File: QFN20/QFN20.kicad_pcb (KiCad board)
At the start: 2 copper layers, 25.7 x 13 mm, 9 parts, among them J1 Conn_01x10, J2 Conn_02x10_Counter_Clockwise, J3 Conn_01x10, J4 Conn_02x10_Counter_Clockwise, J5 Conn_01x03

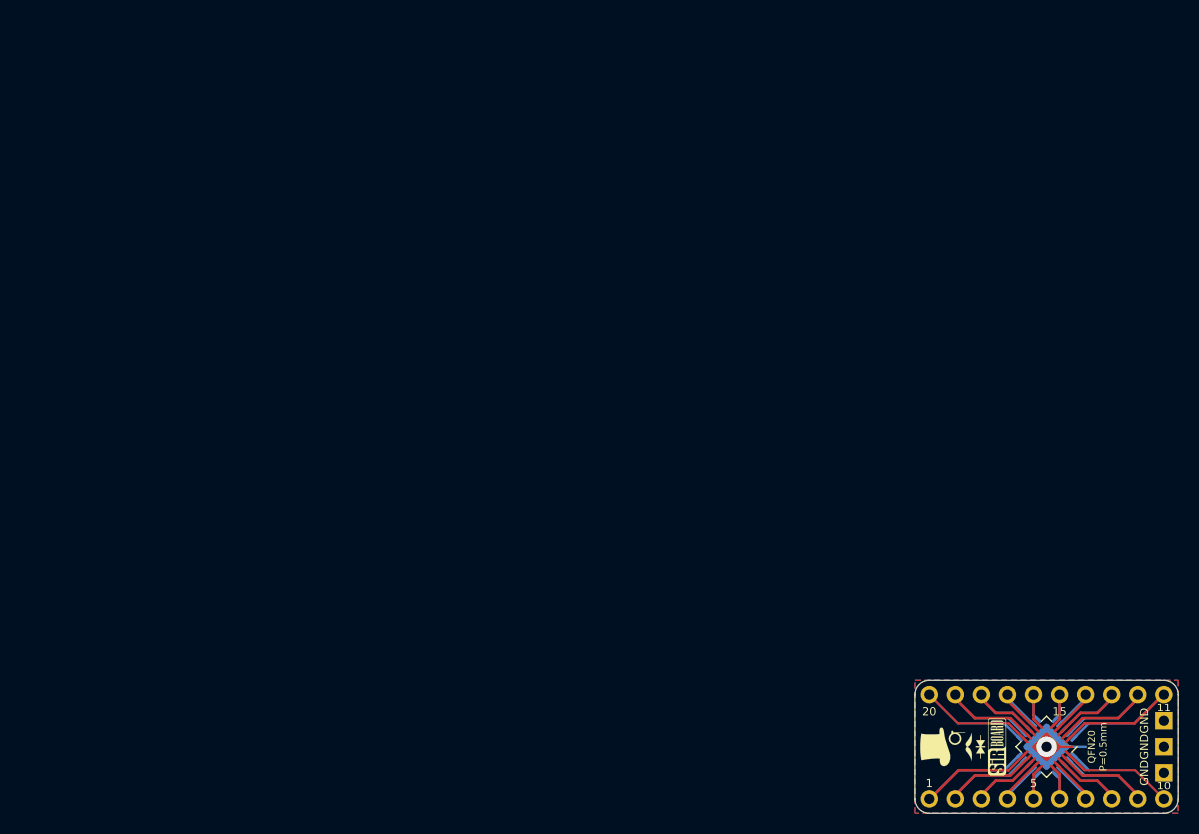
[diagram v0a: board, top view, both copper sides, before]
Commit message: Page Settings Updated
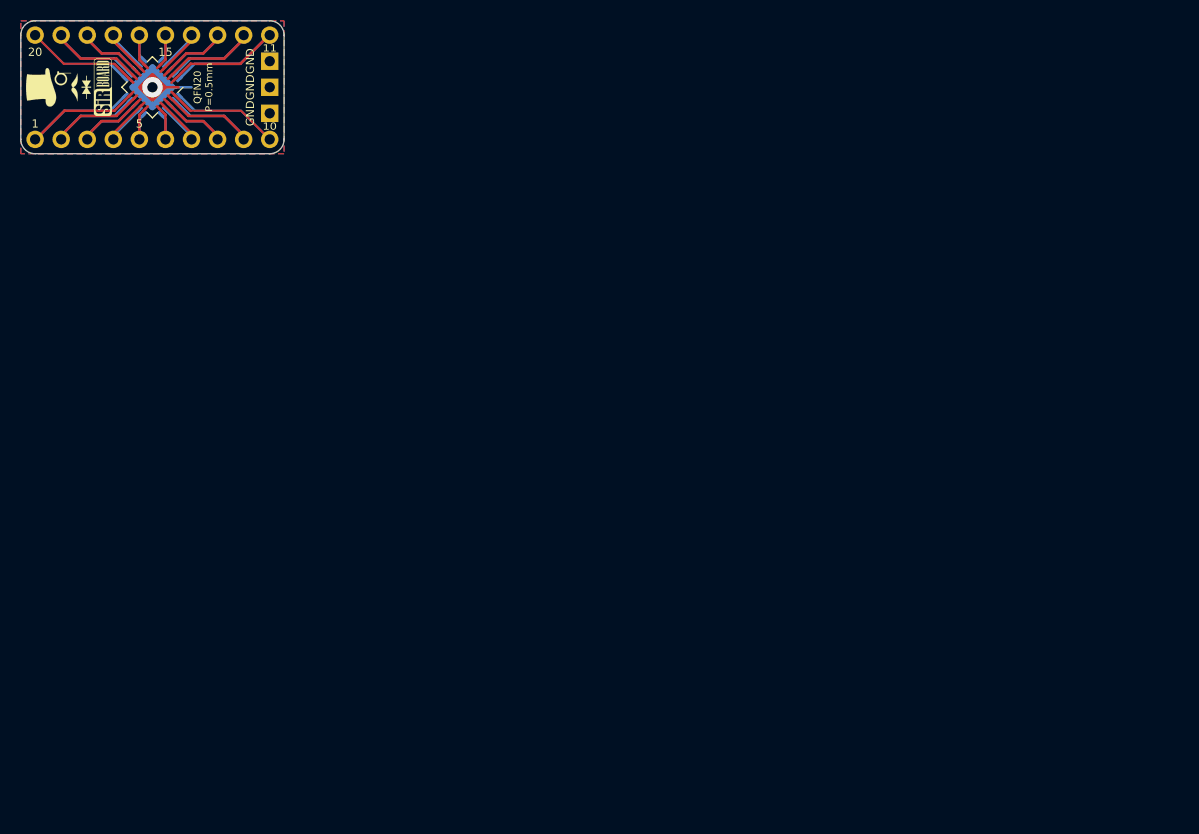
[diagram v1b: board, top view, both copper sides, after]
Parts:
- moved G*** 108.3 mm to (61.2, 42.2)
- moved G*** 108.3 mm to (61.1, 42.0)
- moved G*** 108.3 mm to (65.5, 42.2) (x2)
- moved J1 108.3 mm to (81.8, 37.1)
- moved J3 108.3 mm to (81.8, 47.2)
- moved J5 108.3 mm to (81.8, 39.6)
- moved J2 108.3 mm to (70.4, 42.2)
- moved J4 108.3 mm to (70.4, 42.2)

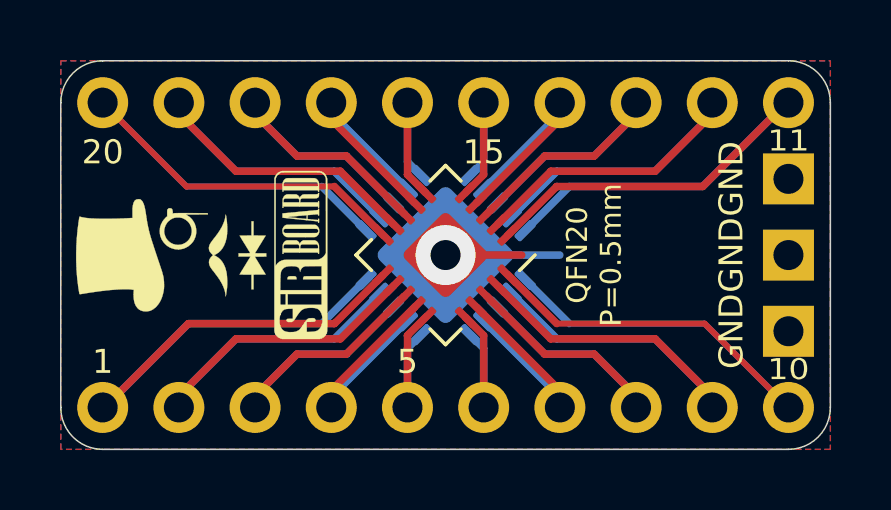
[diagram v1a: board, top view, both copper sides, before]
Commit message: Board Updates
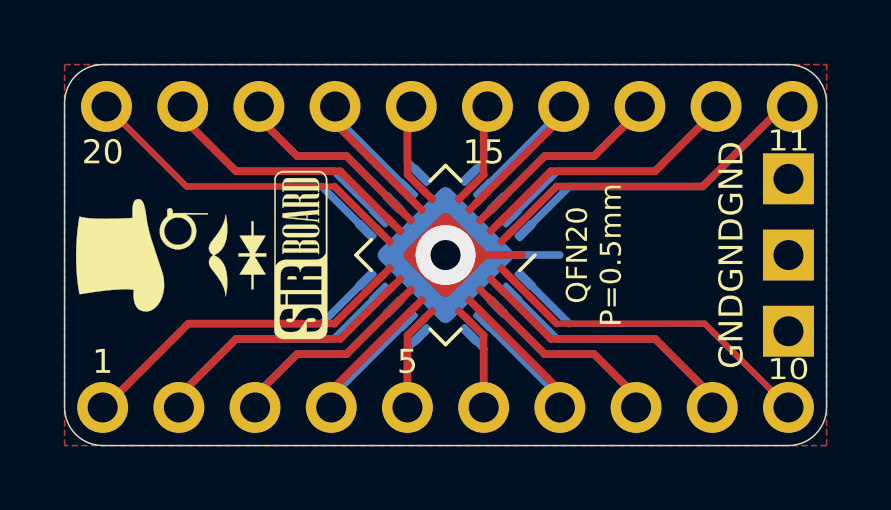
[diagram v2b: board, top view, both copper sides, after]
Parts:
- moved J1 0.18 mm to (81.9, 37.2)
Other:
- board size 25.7 x 13 mm -> 25.4 x 12.7 mm
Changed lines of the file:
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@@
   )
   (module Connector_PinHeader_2.54mm:PinHeader_1x10_P2.54mm_Vertical (layer F.Cu)
-    (at 81.788 37.084 270)
+    (at 81.915 37.211 270)
     (descr "Through hole straight pin header, 1x10, 2.54mm pitch, single row")
     (tags "Through hole pin header THT 1x10 2.54mm single row")
@@
     )
   )
+  (gr_arc (start 81.788 37.084) (end 83.058 37.084) (angle -90) (layer Edge.Cuts) (width 0.05))
+  (gr_arc (start 81.788 47.244) (end 81.788 48.514) (angle -90) (layer Edge.Cuts) (width 0.05))
+  (gr_arc (start 58.928 47.244) (end 57.658 47.244) (angle -90) (layer Edge.Cuts) (width 0.05))
+  (gr_arc (start 58.928 37.084) (end 58.928 35.814) (angle -90) (layer Edge.Cuts) (width 0.05))
   (dimension 22.86 (width 0.15) (layer Dwgs.User)
     (gr_text "22.860 mm" (at 70.358 32.609) (layer Dwgs.User)
@@
     (arrow2b (pts (xy 58.928 33.909) (xy 60.054504 33.322579)))
   )
-  (dimension 25.654 (width 0.15) (layer Dwgs.User)
-    (gr_text "25.654 mm" (at 70.358 29.942) (layer Dwgs.User)
+  (dimension 25.4 (width 0.15) (layer Dwgs.User)
+    (gr_text "25.400 mm" (at 70.358 30.069) (layer Dwgs.User)
       (effects (font (size 1 1) (thickness 0.15)) hide)
     )
-    (feature1 (pts (xy 83.185 35.687) (xy 83.185 30.655579)))
-    (feature2 (pts (xy 57.531 35.687) (xy 57.531 30.655579)))
-    (crossbar (pts (xy 57.531 31.242) (xy 83.185 31.242)))
-    (arrow1a (pts (xy 83.185 31.242) (xy 82.058496 31.828421)))
-    (arrow1b (pts (xy 83.185 31.242) (xy 82.058496 30.655579)))
-    (arrow2a (pts (xy 57.531 31.242) (xy 58.657504 31.828421)))
-    (arrow2b (pts (xy 57.531 31.242) (xy 58.657504 30.655579)))
+    (feature1 (pts (xy 83.058 37.084) (xy 83.058 30.782579)))
+    (feature2 (pts (xy 57.658 37.084) (xy 57.658 30.782579)))
+    (crossbar (pts (xy 57.658 31.369) (xy 83.058 31.369)))
+    (arrow1a (pts (xy 83.058 31.369) (xy 81.931496 31.955421)))
+    (arrow1b (pts (xy 83.058 31.369) (xy 81.931496 30.782579)))
+    (arrow2a (pts (xy 57.658 31.369) (xy 58.784504 31.955421)))
+    (arrow2b (pts (xy 57.658 31.369) (xy 58.784504 30.782579)))
   )
   (gr_text 11 (at 81.788 45.974 180) (layer B.SilkS)
@@
     (arrow2b (pts (xy 55.372 47.244) (xy 54.785579 46.117496)))
   )
-  (dimension 12.954 (width 0.15) (layer Dwgs.User)
-    (gr_text "12.954 mm" (at 50.77 42.164 90) (layer Dwgs.User)
+  (dimension 12.7 (width 0.15) (layer Dwgs.User)
+    (gr_text "12.700 mm" (at 51.278 42.164 90) (layer Dwgs.User)
       (effects (font (size 1 1) (thickness 0.15)) hide)
     )
-    (feature1 (pts (xy 57.531 35.687) (xy 51.483579 35.687)))
-    (feature2 (pts (xy 57.531 48.641) (xy 51.483579 48.641)))
-    (crossbar (pts (xy 52.07 48.641) (xy 52.07 35.687)))
-    (arrow1a (pts (xy 52.07 35.687) (xy 52.656421 36.813504)))
-    (arrow1b (pts (xy 52.07 35.687) (xy 51.483579 36.813504)))
-    (arrow2a (pts (xy 52.07 48.641) (xy 52.656421 47.514496)))
-    (arrow2b (pts (xy 52.07 48.641) (xy 51.483579 47.514496)))
+    (feature1 (pts (xy 58.928 35.814) (xy 51.991579 35.814)))
+    (feature2 (pts (xy 58.928 48.514) (xy 51.991579 48.514)))
+    (crossbar (pts (xy 52.578 48.514) (xy 52.578 35.814)))
+    (arrow1a (pts (xy 52.578 35.814) (xy 53.164421 36.940504)))
+    (arrow1b (pts (xy 52.578 35.814) (xy 51.991579 36.940504)))
+    (arrow2a (pts (xy 52.578 48.514) (xy 53.164421 47.387496)))
+    (arrow2b (pts (xy 52.578 48.514) (xy 51.991579 47.387496)))
   )
   (gr_text GND (at 79.883 44.704 90) (layer B.SilkS)
@@
     (effects (font (size 0.7 0.7) (thickness 0.15)))
   )
-  (gr_line (start 57.531 37.084) (end 57.531 47.244) (layer Edge.Cuts) (width 0.05))
-  (gr_line (start 81.788 35.687) (end 58.928 35.687) (layer Edge.Cuts) (width 0.05))
-  (gr_line (start 83.185 47.244) (end 83.185 37.084) (layer Edge.Cuts) (width 0.05))
-  (gr_line (start 58.928 48.641) (end 81.788 48.641) (layer Edge.Cuts) (width 0.05))
-  (gr_arc (start 58.928 47.244) (end 57.531 47.244) (angle -90) (layer Edge.Cuts) (width 0.05))
-  (gr_arc (start 58.928 37.084) (end 58.928 35.687) (angle -90) (layer Edge.Cuts) (width 0.05))
-  (gr_arc (start 81.788 37.084) (end 83.185 37.084) (angle -90) (layer Edge.Cuts) (width 0.05))
-  (gr_arc (start 81.788 47.244) (end 81.788 48.641) (angle -90) (layer Edge.Cuts) (width 0.05))
+  (gr_line (start 57.658 37.084) (end 57.658 47.244) (layer Edge.Cuts) (width 0.05))
+  (gr_line (start 81.788 35.814) (end 58.928 35.814) (layer Edge.Cuts) (width 0.05))
+  (gr_line (start 83.058 47.244) (end 83.058 37.084) (layer Edge.Cuts) (width 0.05))
+  (gr_line (start 58.928 48.514) (end 81.788 48.514) (layer Edge.Cuts) (width 0.05))
   (segment (start 68.280874 41.506204) (end 66.65267 39.878) (width 0.25) (layer F.Cu) (net 1))
   (segment (start 67.70635 41.350827) (end 66.233523 39.878) (width 0.25) (layer B.Cu) (net 1))
@@
     (polygon
       (pts
-        (xy 57.531 48.641) (xy 57.531 35.687) (xy 83.185 35.687) (xy 83.185 48.641)
+        (xy 57.658 48.514) (xy 57.658 35.814) (xy 83.058 35.814) (xy 83.058 48.514)
       )
     )
@@
     (polygon
       (pts
-        (xy 57.531 48.641) (xy 57.531 35.687) (xy 83.185 35.687) (xy 83.185 48.641)
+        (xy 57.658 48.514) (xy 57.658 35.814) (xy 83.058 35.814) (xy 83.058 48.514)
       )
     )
